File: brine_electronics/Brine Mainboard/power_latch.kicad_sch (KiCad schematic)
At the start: 7 parts, among them Q1 AO3407A, U3 LTC2954

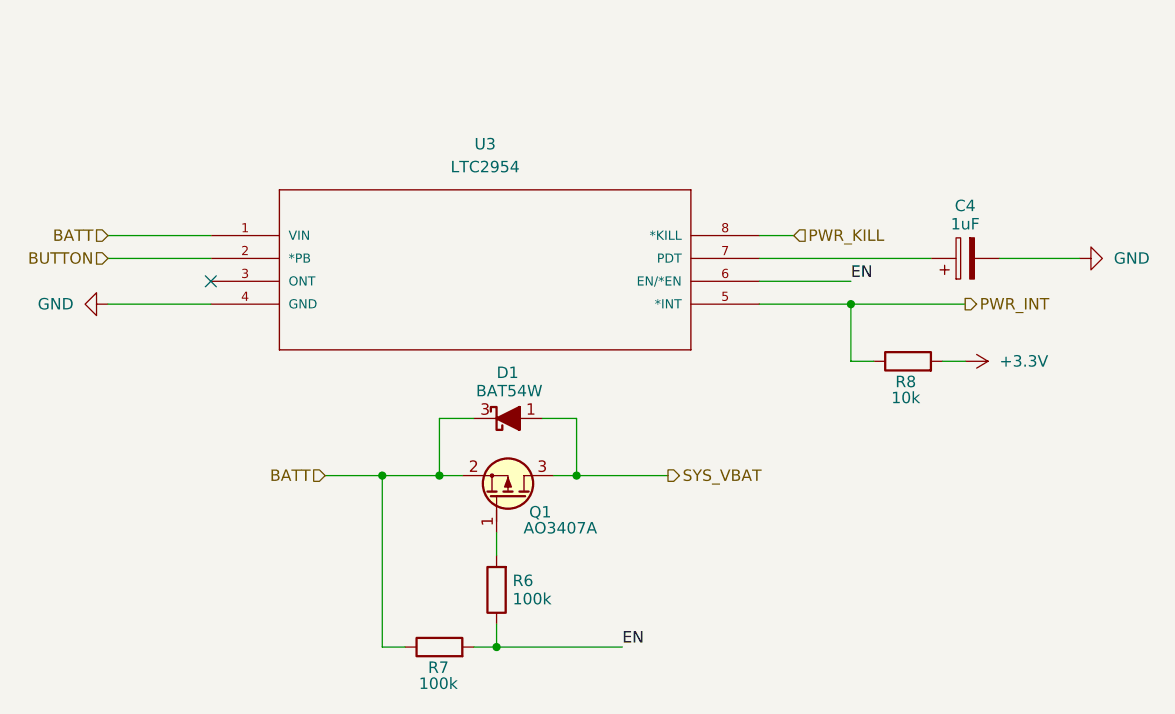
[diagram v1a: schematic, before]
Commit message: Updated button wiring :bug:
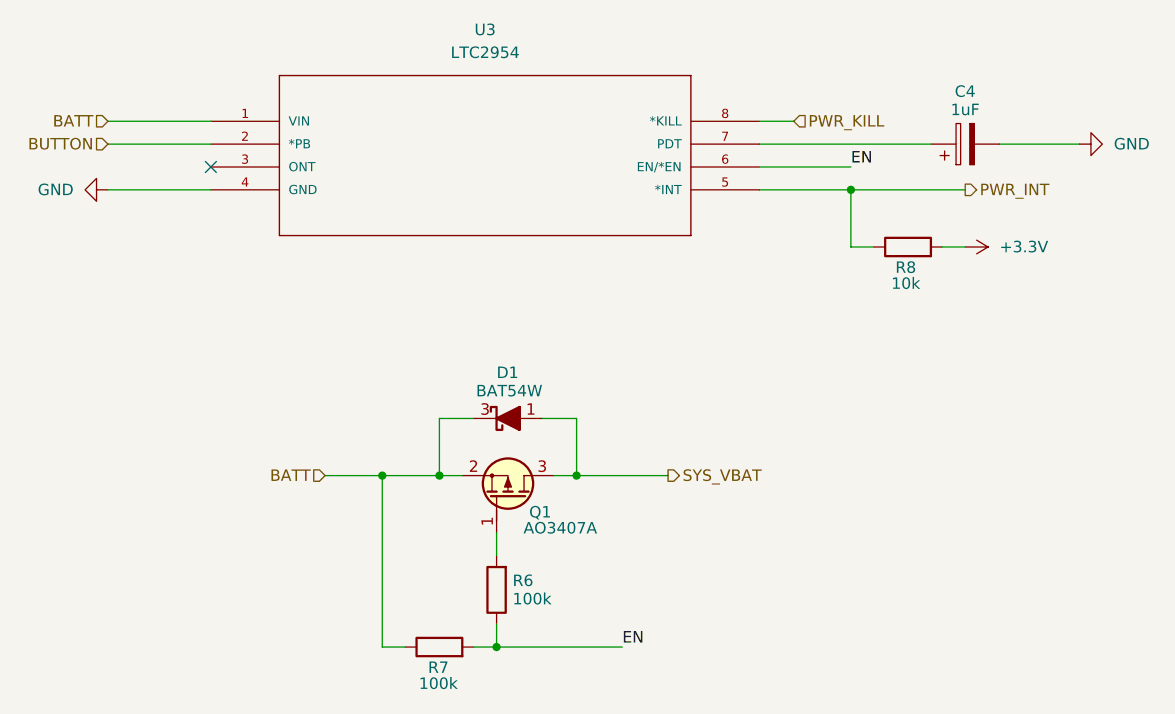
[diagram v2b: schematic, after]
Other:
- moved on the sheet: C4, R8, U3
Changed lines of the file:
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@@
 	)
 	(junction
-		(at 177.8 101.6)
+		(at 177.8 88.9)
 		(diameter 0)
 		(color 0 0 0 0)
@@
 	)
 	(no_connect
-		(at 106.68 99.06)
-	)
-	(wire
-		(pts
-			(xy 194.31 96.52) (xy 203.2 96.52)
+		(at 106.68 86.36)
+	)
+	(wire
+		(pts
+			(xy 194.31 83.82) (xy 203.2 83.82)
 		)
 		(stroke
@@
 	(wire
 		(pts
-			(xy 167.64 99.06) (xy 177.8 99.06)
+			(xy 167.64 86.36) (xy 177.8 86.36)
 		)
 		(stroke
@@
 	(wire
 		(pts
-			(xy 95.25 93.98) (xy 106.68 93.98)
-		)
-		(stroke
-			(width 0)
-			(type default)
-		)
-	)
-	(wire
-		(pts
-			(xy 167.64 101.6) (xy 177.8 101.6)
+			(xy 95.25 81.28) (xy 106.68 81.28)
+		)
+		(stroke
+			(width 0)
+			(type default)
+		)
+	)
+	(wire
+		(pts
+			(xy 167.64 88.9) (xy 177.8 88.9)
 		)
 		(stroke
@@
 	(wire
 		(pts
-			(xy 95.25 96.52) (xy 106.68 96.52)
-		)
-		(stroke
-			(width 0)
-			(type default)
-		)
-	)
-	(wire
-		(pts
-			(xy 180.34 107.95) (xy 177.8 107.95)
+			(xy 95.25 83.82) (xy 106.68 83.82)
+		)
+		(stroke
+			(width 0)
+			(type default)
+		)
+	)
+	(wire
+		(pts
+			(xy 180.34 95.25) (xy 177.8 95.25)
 		)
 		(stroke
@@
 	(wire
 		(pts
-			(xy 167.64 96.52) (xy 186.69 96.52)
+			(xy 167.64 83.82) (xy 186.69 83.82)
 		)
 		(stroke
@@
 	(wire
 		(pts
-			(xy 95.25 101.6) (xy 106.68 101.6)
-		)
-		(stroke
-			(width 0)
-			(type default)
-		)
-	)
-	(wire
-		(pts
-			(xy 167.64 93.98) (xy 171.45 93.98)
+			(xy 95.25 88.9) (xy 106.68 88.9)
+		)
+		(stroke
+			(width 0)
+			(type default)
+		)
+	)
+	(wire
+		(pts
+			(xy 167.64 81.28) (xy 171.45 81.28)
 		)
 		(stroke
@@
 	(wire
 		(pts
-			(xy 187.96 107.95) (xy 190.5 107.95)
+			(xy 187.96 95.25) (xy 190.5 95.25)
 		)
 		(stroke
@@
 	(wire
 		(pts
-			(xy 177.8 101.6) (xy 177.8 107.95)
+			(xy 177.8 88.9) (xy 177.8 95.25)
 		)
 		(stroke
@@
 	(wire
 		(pts
-			(xy 177.8 101.6) (xy 190.5 101.6)
+			(xy 177.8 88.9) (xy 190.5 88.9)
 		)
 		(stroke
@@
 	)
 	(label "EN"
-		(at 177.8 99.06 0)
+		(at 177.8 86.36 0)
 		(effects
 			(font
@@
 	(hierarchical_label "PWR_KILL"
 		(shape input)
-		(at 171.45 93.98 0)
+		(at 171.45 81.28 0)
 		(effects
 			(font
@@
 	(hierarchical_label "BATT"
 		(shape input)
-		(at 95.25 93.98 180)
+		(at 95.25 81.28 180)
 		(effects
 			(font
@@
 	(hierarchical_label "PWR_INT"
 		(shape output)
-		(at 190.5 101.6 0)
+		(at 190.5 88.9 0)
 		(effects
 			(font
@@
 	(hierarchical_label "BUTTON"
 		(shape input)
-		(at 95.25 96.52 180)
+		(at 95.25 83.82 180)
 		(effects
 			(font
@@
 	(symbol
 		(lib_id "PCM_Capacitor_AKL:CP_SMD_Tantalum_Kemet-R_2012")
-		(at 190.5 96.52 90)
+		(at 190.5 83.82 90)
 		(unit 1)
 		(body_style 1)
@@
 		(dnp no)
 		(property "Reference" "C4"
-			(at 190.5 90.678 90)
+			(at 190.5 77.978 90)
 			(show_name no)
 			(do_not_autoplace no)
@@
 		)
 		(property "Value" "1uF"
-			(at 190.5 92.71 90)
+			(at 190.5 80.01 90)
 			(show_name no)
 			(do_not_autoplace no)
@@
 		)
 		(property "Footprint" "PCM_Capacitor_Tantalum_SMD_AKL:CP_EIA-2012-12_Kemet-R"
-			(at 200.66 96.52 0)
+			(at 200.66 83.82 0)
 			(hide yes)
 			(show_name no)
@@
 		)
 		(property "Datasheet" ""
-			(at 190.5 96.52 0)
+			(at 190.5 83.82 0)
 			(hide yes)
 			(show_name no)
@@
 		)
 		(property "Description" "SMD Tantalum Electrolytic Capacitor, Kemet Type R, 2012, European Symbol, Alternate KiCad Library"
-			(at 190.5 96.52 0)
+			(at 190.5 83.82 0)
 			(hide yes)
 			(show_name no)
@@
 	(symbol
 		(lib_id "power:GND")
-		(at 203.2 96.52 90)
+		(at 203.2 83.82 90)
 		(unit 1)
 		(body_style 1)
@@
 		(fields_autoplaced yes)
 		(property "Reference" "#PWR023"
-			(at 209.55 96.52 0)
+			(at 209.55 83.82 0)
 			(hide yes)
 			(show_name no)
@@
 		)
 		(property "Value" "GND"
-			(at 207.01 96.5199 90)
+			(at 207.01 83.8199 90)
 			(show_name no)
 			(do_not_autoplace no)
@@
 		)
 		(property "Footprint" ""
-			(at 203.2 96.52 0)
+			(at 203.2 83.82 0)
 			(hide yes)
 			(show_name no)
@@
 		)
 		(property "Datasheet" ""
-			(at 203.2 96.52 0)
+			(at 203.2 83.82 0)
 			(hide yes)
 			(show_name no)
@@
 		)
 		(property "Description" "Power symbol creates a global label with name \"GND\" , ground"
-			(at 203.2 96.52 0)
+			(at 203.2 83.82 0)
 			(hide yes)
 			(show_name no)
@@
 	(symbol
 		(lib_id "Device:R")
-		(at 184.15 107.95 90)
+		(at 184.15 95.25 90)
 		(unit 1)
 		(body_style 1)
@@
 		(dnp no)
 		(property "Reference" "R8"
-			(at 183.896 110.236 90)
+			(at 183.896 97.536 90)
 			(show_name no)
 			(do_not_autoplace no)
@@
 		)
 		(property "Value" "10k"
-			(at 183.896 112.014 90)
+			(at 183.896 99.314 90)
 			(show_name no)
 			(do_not_autoplace no)
@@
 		)
 		(property "Footprint" "PCM_Resistor_SMD_AKL:R_0805_2012Metric"
-			(at 184.15 109.728 90)
+			(at 184.15 97.028 90)
 			(hide yes)
 			(show_name no)
@@
 		)
 		(property "Datasheet" ""
-			(at 184.15 107.95 0)
+			(at 184.15 95.25 0)
 			(hide yes)
 			(show_name no)
@@
 		)
 		(property "Description" "Resistor"
-			(at 184.15 107.95 0)
+			(at 184.15 95.25 0)
 			(hide yes)
 			(show_name no)
@@
 	(symbol
 		(lib_id "LTC2954CTS8-2_TRMPBF:LTC2954CTS8-2_TRMPBF")
-		(at 106.68 93.98 0)
+		(at 106.68 81.28 0)
 		(unit 1)
 		(body_style 1)
@@
 		(fields_autoplaced yes)
 		(property "Reference" "U3"
-			(at 137.16 83.82 0)
+			(at 137.16 71.12 0)
 			(show_name no)
 			(do_not_autoplace no)
@@
 		)
 		(property "Value" "LTC2954"
-			(at 137.16 86.36 0)
+			(at 137.16 73.66 0)
 			(show_name no)
 			(do_not_autoplace no)
@@
 		)
 		(property "Footprint" "LTC2954CTS8_2_TRMPBF:TSOT-23_TS8"
-			(at 106.68 93.98 0)
+			(at 106.68 81.28 0)
 			(hide yes)
 			(show_name no)
@@
 		)
 		(property "Datasheet" ""
-			(at 106.68 93.98 0)
+			(at 106.68 81.28 0)
 			(hide yes)
 			(show_name no)
@@
 		)
 		(property "Description" ""
-			(at 106.68 93.98 0)
+			(at 106.68 81.28 0)
 			(hide yes)
 			(show_name no)
@@
 		)
 		(property "VENDOR" "Linear Technology"
-			(at 106.68 93.98 0)
+			(at 106.68 81.28 0)
 			(hide yes)
 			(show_name no)
@@
 		)
 		(property "MANUFACTURER_PART_NUMBER" "ltc2954cts81"
-			(at 106.68 93.98 0)
+			(at 106.68 81.28 0)
 			(hide yes)
 			(show_name no)
@@
 		)
 		(property "DigiKey Link" "https://www.digikey.com/en/products/detail/analog-devices-inc/LTC2954CTS8-2-TRMPBF/1232658"
-			(at 106.68 93.98 0)
+			(at 106.68 81.28 0)
 			(hide yes)
 			(show_name no)
@@
 	(symbol
 		(lib_id "power:GND")
-		(at 95.25 101.6 270)
+		(at 95.25 88.9 270)
 		(unit 1)
 		(body_style 1)
@@
 		(fields_autoplaced yes)
 		(property "Reference" "#PWR08"
-			(at 88.9 101.6 0)
+			(at 88.9 88.9 0)
 			(hide yes)
 			(show_name no)
@@
 		)
 		(property "Value" "GND"
-			(at 91.44 101.5999 90)
+			(at 91.44 88.8999 90)
 			(show_name no)
 			(do_not_autoplace no)
@@
 		)
 		(property "Footprint" ""
-			(at 95.25 101.6 0)
+			(at 95.25 88.9 0)
 			(hide yes)
 			(show_name no)
@@
 		)
 		(property "Datasheet" ""
-			(at 95.25 101.6 0)
+			(at 95.25 88.9 0)
 			(hide yes)
 			(show_name no)
@@
 		)
 		(property "Description" "Power symbol creates a global label with name \"GND\" , ground"
-			(at 95.25 101.6 0)
+			(at 95.25 88.9 0)
 			(hide yes)
 			(show_name no)
@@
 	(symbol
 		(lib_id "power:+3.3V")
-		(at 190.5 107.95 270)
+		(at 190.5 95.25 270)
 		(unit 1)
 		(body_style 1)
@@
 		(fields_autoplaced yes)
 		(property "Reference" "#PWR025"
-			(at 186.69 107.95 0)
+			(at 186.69 95.25 0)
 			(hide yes)
 			(show_name no)
@@
 		)
 		(property "Value" "+3.3V"
-			(at 194.31 107.9499 90)
+			(at 194.31 95.2499 90)
 			(show_name no)
 			(do_not_autoplace no)
@@
 		)
 		(property "Footprint" ""
-			(at 190.5 107.95 0)
+			(at 190.5 95.25 0)
 			(hide yes)
 			(show_name no)
@@
 		)
 		(property "Datasheet" ""
-			(at 190.5 107.95 0)
+			(at 190.5 95.25 0)
 			(hide yes)
 			(show_name no)
@@
 		)
 		(property "Description" "Power symbol creates a global label with name \"+3.3V\""
-			(at 190.5 107.95 0)
-			(hide yes)
-			(show_name no)
+			(at 190.5 95.25 0)
+			(hide yes)
+			(show_name no)

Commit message: Updated production files 🏭
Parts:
- C4: LCSC Part # (none) -> C1952822
- D1: LCSC Part # (none) -> C8657
- Q1: LCSC Part # (none) -> C347478
- R6, R7: LCSC Part # (none) -> C25611
- R8: LCSC Part # (none) -> C17414
- U3: LCSC Part # (none) -> C580656
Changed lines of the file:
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@@
+			)
+		)
+		(property "Color" ""
+			(at 190.5 83.82 90)
+			(hide yes)
+			(show_name no)
+			(do_not_autoplace no)
+			(effects
+				(font
+					(size 1.27 1.27)
+				)
+			)
+		)
+		(property "LCSC Part #" "C1952822"
+			(at 190.5 83.82 90)
+			(hide yes)
+			(show_name no)
+			(do_not_autoplace no)
+			(effects
+				(font
+					(size 1.27 1.27)
+				)
 			)
 		)
@@
 			)
 		)
+		(property "Color" ""
+			(at 139.7 114.3 0)
+			(hide yes)
+			(show_name no)
+			(do_not_autoplace no)
+			(effects
+				(font
+					(size 1.27 1.27)
+				)
+			)
+		)
+		(property "LCSC Part #" "C8657"
+			(at 139.7 114.3 0)
+			(hide yes)
+			(show_name no)
+			(do_not_autoplace no)
+			(effects
+				(font
+					(size 1.27 1.27)
+				)
+			)
+		)
 		(pin "3"
 		)
@@
 			)
 		)
+		(property "Color" ""
+			(at 132.08 139.7 90)
+			(hide yes)
+			(show_name no)
+			(do_not_autoplace no)
+			(effects
+				(font
+					(size 1.27 1.27)
+				)
+			)
+		)
+		(property "LCSC Part #" "C25611"
+			(at 132.08 139.7 90)
+			(hide yes)
+			(show_name no)
+			(do_not_autoplace no)
+			(effects
+				(font
+					(size 1.27 1.27)
+				)
+			)
+		)
 		(pin "1"
 		)
@@
 			)
 		)
+		(property "Color" ""
+			(at 139.7 123.19 90)
+			(hide yes)
+			(show_name no)
+			(do_not_autoplace no)
+			(effects
+				(font
+					(size 1.27 1.27)
+				)
+			)
+		)
+		(property "LCSC Part #" "C347478"
+			(at 139.7 123.19 90)
+			(hide yes)
+			(show_name no)
+			(do_not_autoplace no)
+			(effects
+				(font
+					(size 1.27 1.27)
+				)
+			)
+		)
 		(pin "1"
 		)
@@
 			)
 		)
+		(property "Color" ""
+			(at 184.15 95.25 90)
+			(hide yes)
+			(show_name no)
+			(do_not_autoplace no)
+			(effects
+				(font
+					(size 1.27 1.27)
+				)
+			)
+		)
+		(property "LCSC Part #" "C17414"
+			(at 184.15 95.25 90)
+			(hide yes)
+			(show_name no)
+			(do_not_autoplace no)
+			(effects
+				(font
+					(size 1.27 1.27)
+				)
+			)
+		)
 		(pin "1"
 		)
@@
 		)
 		(property "Description" "Resistor"
+			(at 138.43 133.35 0)
+			(hide yes)
+			(show_name no)
+			(do_not_autoplace no)
+			(effects
+				(font
+					(size 1.27 1.27)
+				)
+			)
+		)
+		(property "Color" ""
+			(at 138.43 133.35 0)
+			(hide yes)
+			(show_name no)
+			(do_not_autoplace no)
+			(effects
+				(font
+					(size 1.27 1.27)
+				)
+			)
+		)
+		(property "LCSC Part #" "C25611"
 			(at 138.43 133.35 0)
 			(hide yes)
@@
 			(at 106.68 81.28 0)
 			(hide yes)
+			(show_name no)
+			(do_not_autoplace no)
+			(effects
+				(font
+					(size 1.27 1.27)
+				)
+			)
+		)
+		(property "Color" ""
+			(at 106.68 81.28 0)
+			(hide yes)
+			(show_name no)
+			(do_not_autoplace no)
+			(effects
+				(font
+					(size 1.27 1.27)
+				)
+			)
+		)
+		(property "LCSC Part #" "C580656"
+			(at 106.68 81.28 0)
+			(hide yes)

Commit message: Updated electronics production files 🏭
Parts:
- C4: JLCPCB Part # (none) -> C1952822; LCSC Part # C1952822 -> (none)
- D1: JLCPCB Part # (none) -> C8657; LCSC Part # C8657 -> (none)
- Q1: JLCPCB Part # (none) -> C347478; LCSC Part # C347478 -> (none)
- R6, R7: JLCPCB Part # (none) -> C25611; LCSC Part # C25611 -> (none)
- R8: JLCPCB Part # (none) -> C17414; LCSC Part # C17414 -> (none)
- U3: JLCPCB Part # (none) -> C580656; LCSC Part # C580656 -> (none)
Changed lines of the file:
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@@
 			)
 		)
-		(property "LCSC Part #" "C1952822"
+		(property "JLCPCB Part #" "C1952822"
 			(at 190.5 83.82 90)
 			(hide yes)
@@
 			)
 		)
-		(property "LCSC Part #" "C8657"
+		(property "JLCPCB Part #" "C8657"
 			(at 139.7 114.3 0)
 			(hide yes)
@@
 			)
 		)
-		(property "LCSC Part #" "C25611"
+		(property "JLCPCB Part #" "C25611"
 			(at 132.08 139.7 90)
 			(hide yes)
@@
 			)
 		)
-		(property "LCSC Part #" "C347478"
+		(property "JLCPCB Part #" "C347478"
 			(at 139.7 123.19 90)
 			(hide yes)
@@
 			)
 		)
-		(property "LCSC Part #" "C17414"
+		(property "JLCPCB Part #" "C17414"
 			(at 184.15 95.25 90)
 			(hide yes)
@@
 			)
 		)
-		(property "LCSC Part #" "C25611"
+		(property "JLCPCB Part #" "C25611"
 			(at 138.43 133.35 0)
 			(hide yes)
@@
 			)
 		)
-		(property "LCSC Part #" "C580656"
+		(property "JLCPCB Part #" "C580656"
 			(at 106.68 81.28 0)
 			(hide yes)
